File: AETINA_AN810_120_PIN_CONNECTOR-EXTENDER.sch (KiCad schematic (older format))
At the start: 4 parts, among them J1 QTH-060-01-X-D-A, J2 QSH-060-01-X-D-A

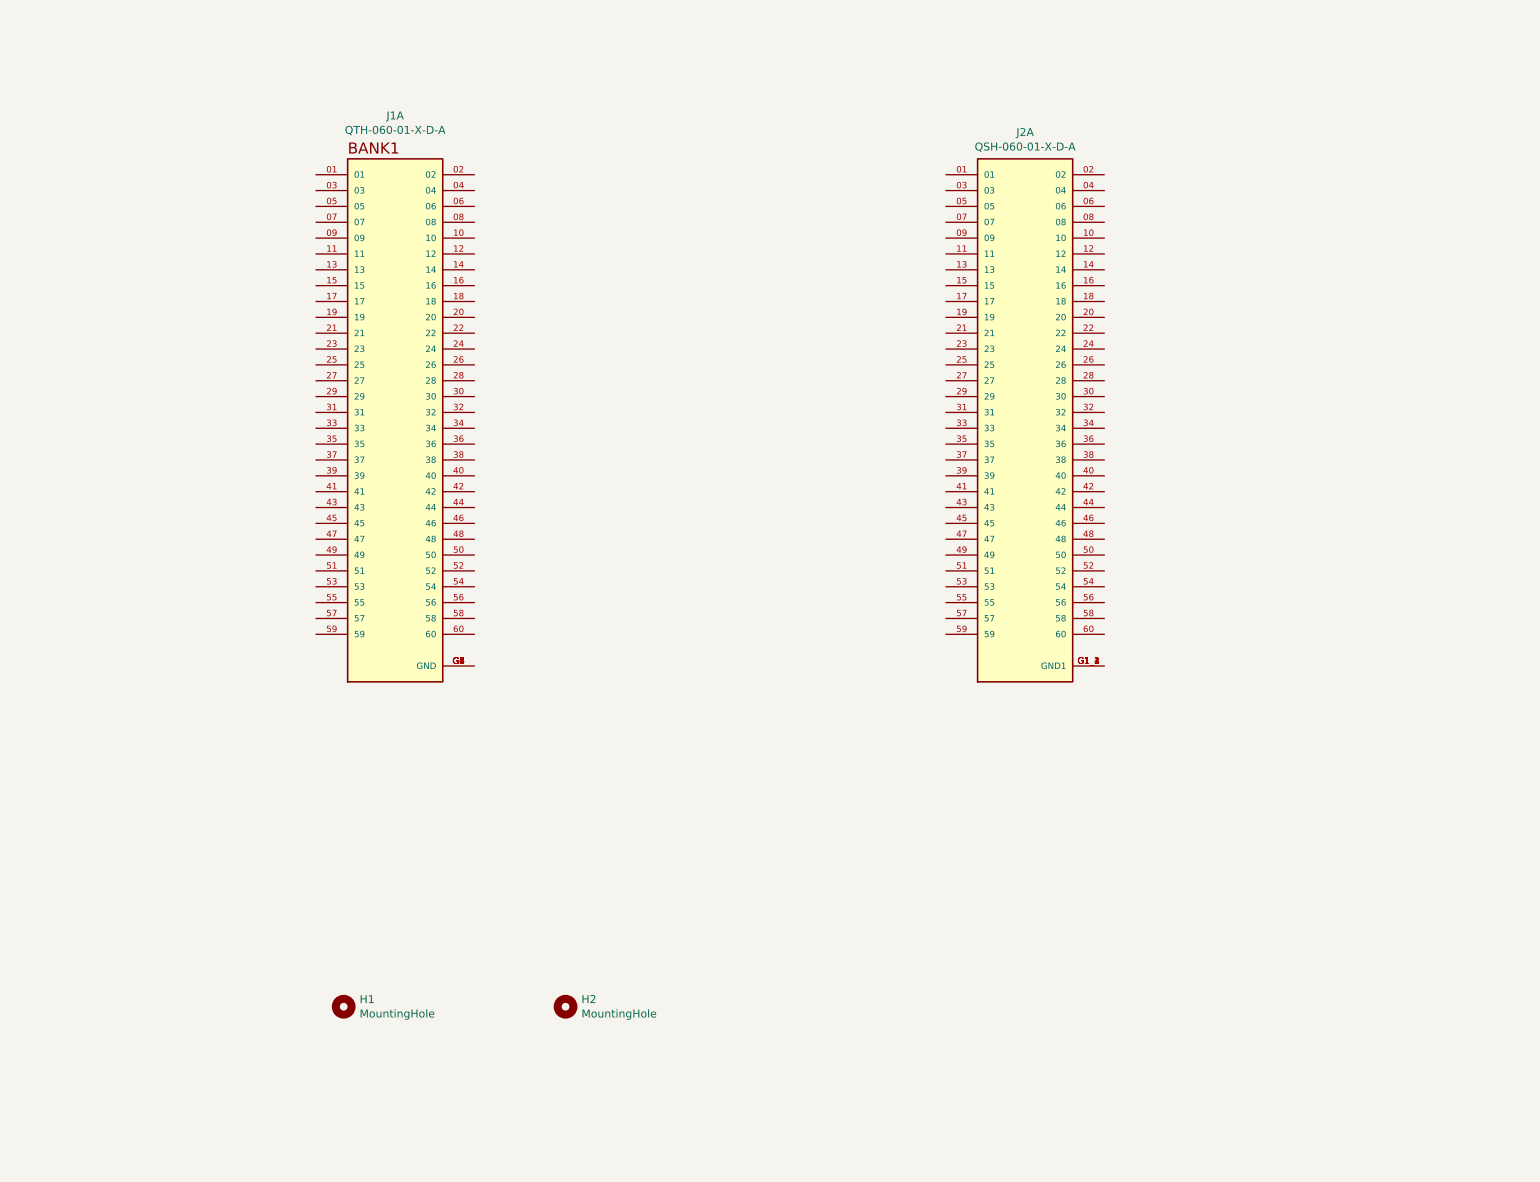
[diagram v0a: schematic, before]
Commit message: Routing completed
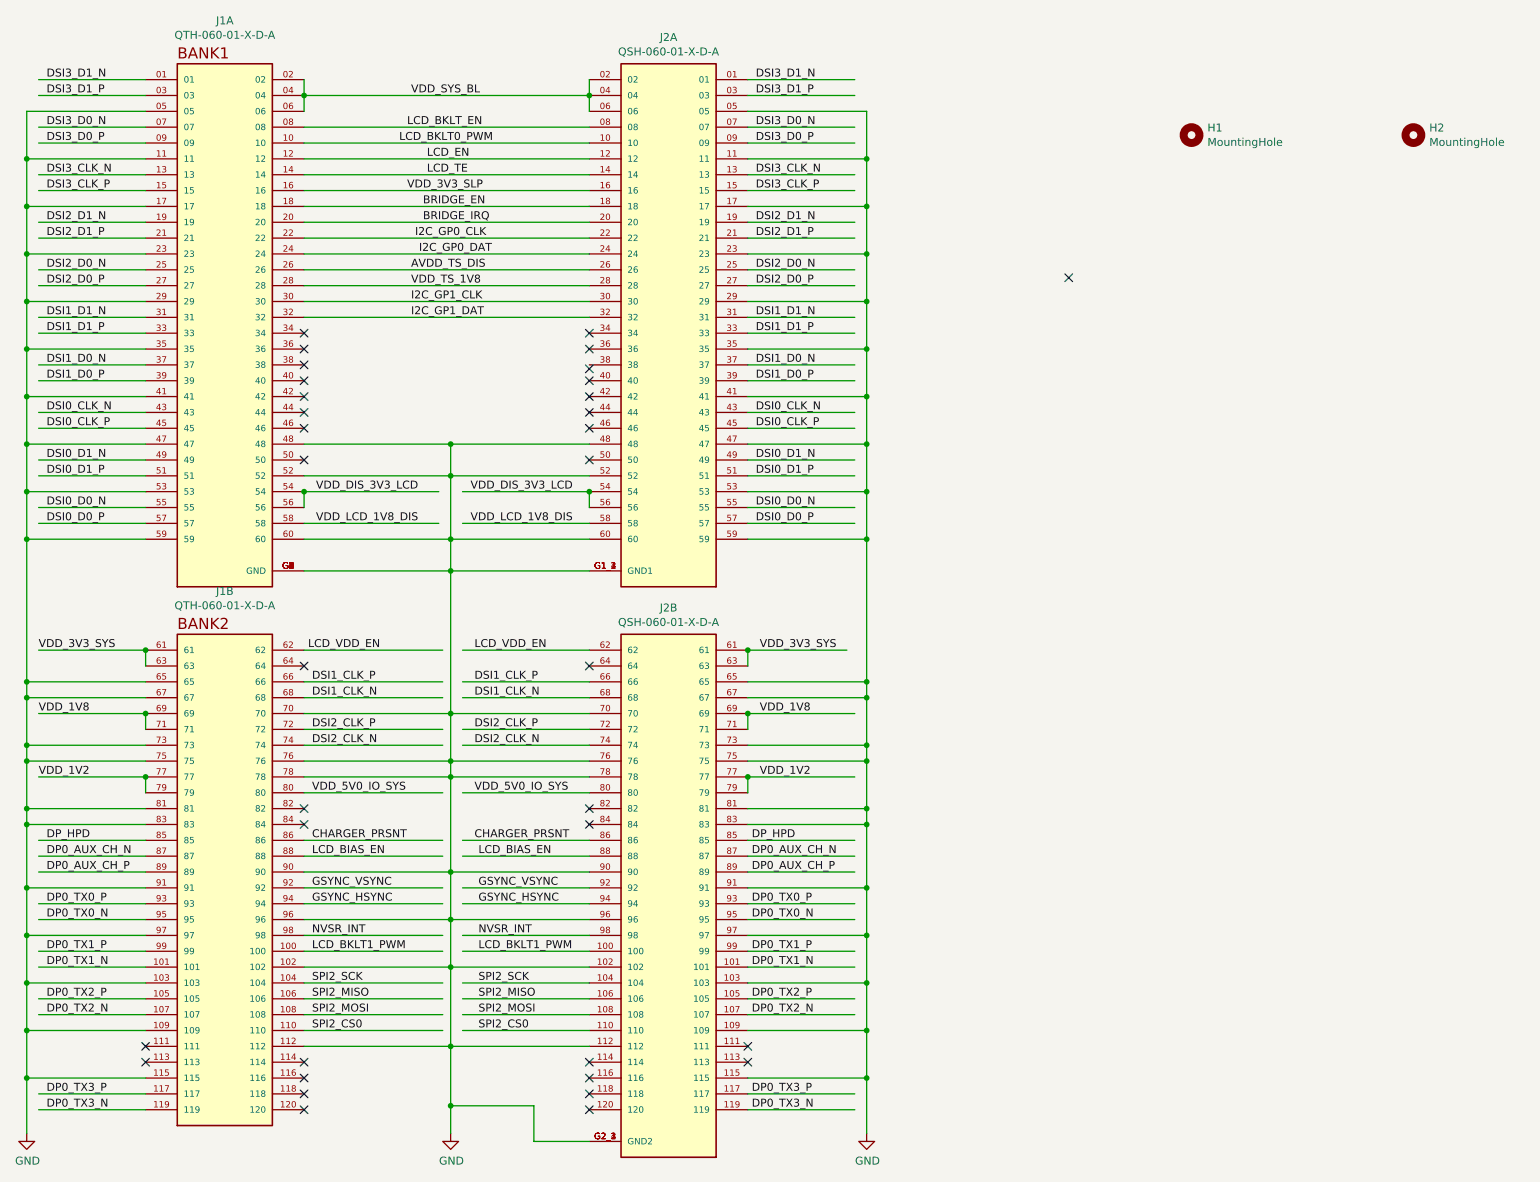
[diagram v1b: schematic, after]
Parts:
- added unit 2 of J1
- added unit 2 of J2
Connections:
- net labels added: AVDD_TS_DIS, BRIDGE_EN, BRIDGE_IRQ, CHARGER_PRSNT, DP0_AUX_CH_N, DP0_AUX_CH_P, DP0_TX0_N, DP0_TX0_P, DP0_TX1_N, DP0_TX1_P, DP0_TX2_N, DP0_TX2_P, DP0_TX3_N, DP0_TX3_P, DP_HPD, DSI0_CLK_N, DSI0_CLK_P, DSI0_D0_N, DSI0_D0_P, DSI0_D1_N, DSI0_D1_P, DSI1_CLK_N, DSI1_CLK_P, DSI1_D0_N, DSI1_D0_P, DSI1_D1_N, DSI1_D1_P, DSI2_CLK_N, DSI2_CLK_P, DSI2_D0_N, DSI2_D0_P, DSI2_D1_N, DSI2_D1_P, DSI3_CLK_N, DSI3_CLK_P, DSI3_D0_N, DSI3_D0_P, DSI3_D1_N, DSI3_D1_P, GND, GSYNC_HSYNC, GSYNC_VSYNC, I2C_GP0_CLK, I2C_GP0_DAT, I2C_GP1_CLK, I2C_GP1_DAT, LCD_BIAS_EN, LCD_BKLT0_PWM, LCD_BKLT1_PWM, LCD_BKLT_EN, LCD_EN, LCD_TE, LCD_VDD_EN, NVSR_INT, SPI2_CS0, SPI2_MISO, SPI2_MOSI, SPI2_SCK, VDD_1V2, VDD_1V8, VDD_3V3_SLP, VDD_3V3_SYS, VDD_5V0_IO_SYS, VDD_DIS_3V3_LCD, VDD_LCD_1V8_DIS, VDD_SYS_BL, VDD_TS_1V8
- wire segments 0 -> 251
- no-connect marks 0 -> 35
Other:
- moved on the sheet: H1, H2, J1A, J2A
